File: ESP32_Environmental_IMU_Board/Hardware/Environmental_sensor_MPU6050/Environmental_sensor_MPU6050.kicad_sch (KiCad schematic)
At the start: 63 parts, among them J1 Conn_01x04_Pin, J2 Conn_01x04_Pin, J3 USB_C_Receptacle_USB2.0_16P, J4 Micro_SD_Card, SW1 SW_Push, SW2 SW_Push, U1 MPU-6050, U2 AP2112K-3.3, U3 USBLC6-2P6, U4 ESP32-S3-WROOM-1, U5 BME280, U6 DS3231M

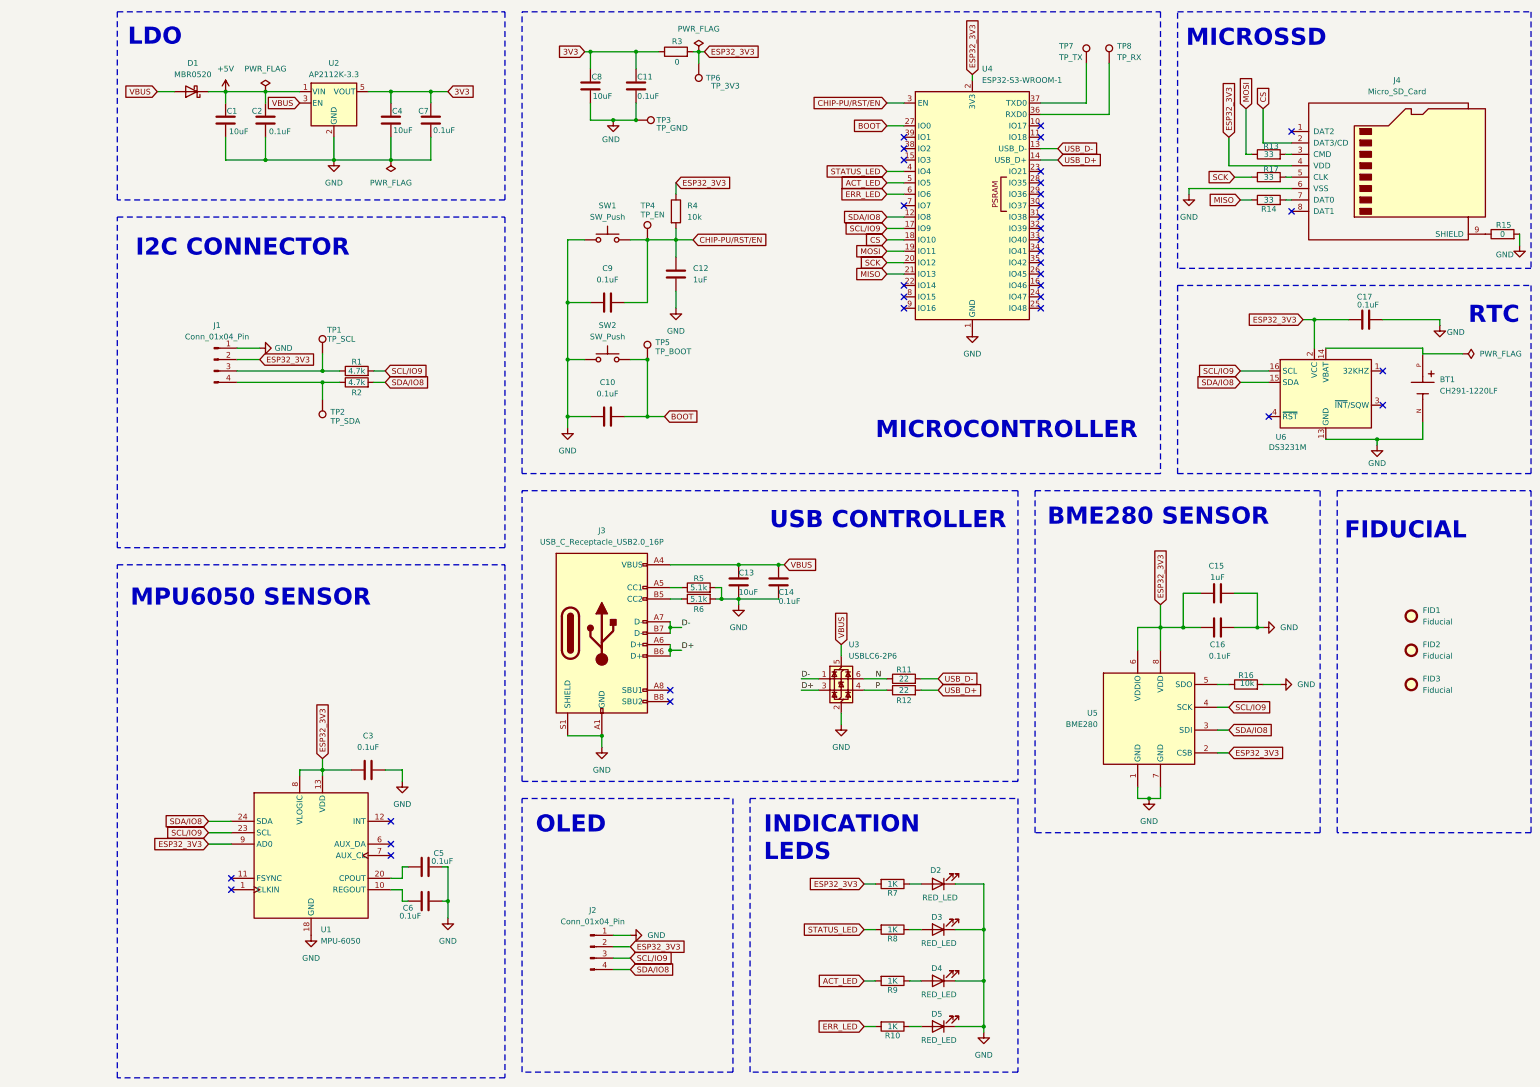
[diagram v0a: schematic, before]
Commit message: Schematic reaaranged, Board setup loaded
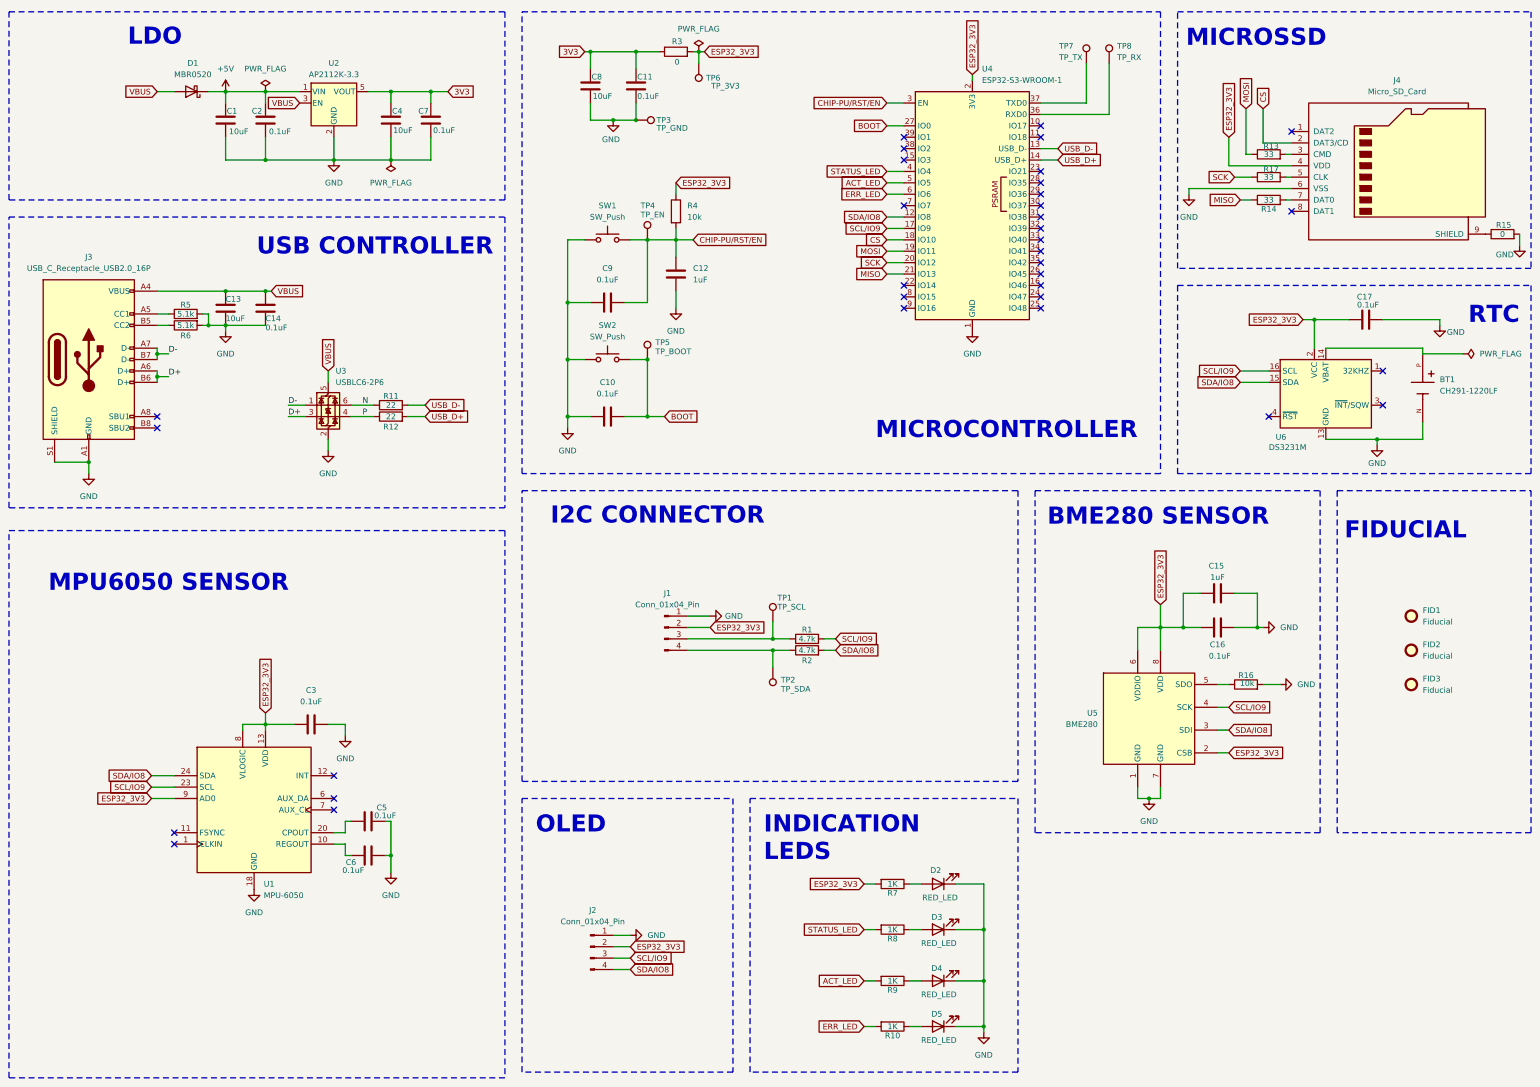
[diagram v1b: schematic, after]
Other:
- moved on the sheet: C13, C14, C3, C5, C6, J1, J3, R1, R11, R12, R2, R5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
